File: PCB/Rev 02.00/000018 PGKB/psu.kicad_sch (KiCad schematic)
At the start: 12 parts, among them U6 MCP1825T-3302E/DC, U7 CAT811TTBI-GT3

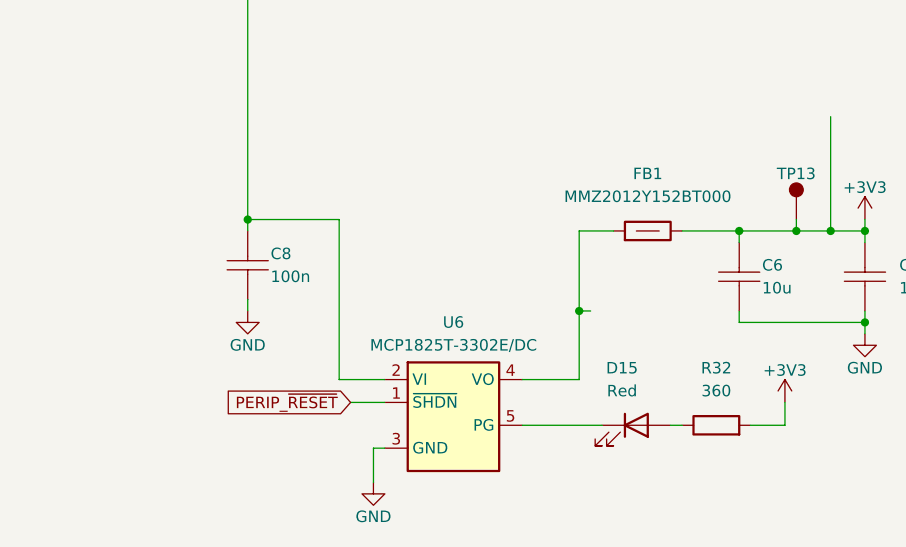
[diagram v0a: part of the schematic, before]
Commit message: Leiskaa
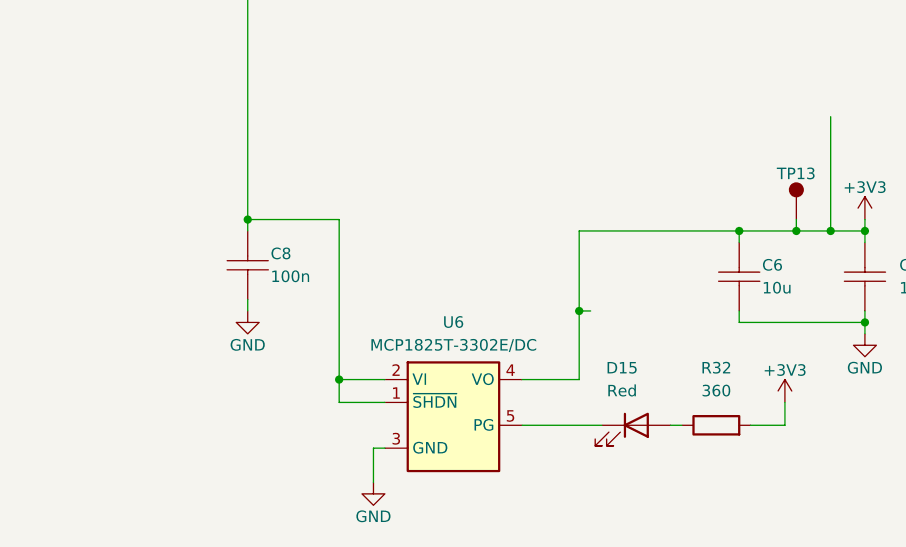
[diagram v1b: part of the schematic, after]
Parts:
- removed FB1: Ferrite_500mA_TDK_MMZ2012Y152BT000, KD_Inductor:INDC2016X100N, symbol KD_Inductor:Ferrite_500mA_TDK_MMZ2012Y152BT000
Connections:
- net +3V3: now also U6.4 (VO)
- net PERIP_~{RESET}: no longer U6.1 (~{SHDN})
- net PWR_IN: now also U6.1 (~{SHDN})
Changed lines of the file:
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@@
   (junction (at 214.63 111.76) (diameter 0) (color 0 0 0 0)
   )
+  (junction (at 81.28 128.27) (diameter 0) (color 0 0 0 0)
+  )
   (junction (at 180.34 111.76) (diameter 0) (color 0 0 0 0)
   )
@@
     (stroke (width 0) (type default))
   )
+  (wire (pts (xy 81.28 130.81) (xy 81.28 128.27))
+    (stroke (width 0) (type default))
+  )
   (wire (pts (xy 81.28 128.27) (xy 86.36 128.27))
     (stroke (width 0) (type default))
@@
     (stroke (width 0) (type default))
   )
-  (wire (pts (xy 82.55 130.81) (xy 86.36 130.81))
+  (wire (pts (xy 81.28 130.81) (xy 86.36 130.81))
     (stroke (width 0) (type default))
   )
@@
     (stroke (width 0) (type default))
   )
-  (wire (pts (xy 119.38 111.76) (xy 125.73 111.76))
-    (stroke (width 0) (type default))
-  )
   (wire (pts (xy 101.6 133.35) (xy 110.49 133.35))
     (stroke (width 0) (type default))
@@
     (stroke (width 0) (type default))
   )
-  (wire (pts (xy 107.95 111.76) (xy 111.76 111.76))
+  (wire (pts (xy 107.95 111.76) (xy 125.73 111.76))
     (stroke (width 0) (type default))
   )
@@
   (wire (pts (xy 139.7 113.03) (xy 139.7 111.76))
     (stroke (width 0) (type default))
-  )
-  (global_label "PERIP_~{RESET}" (shape input) (at 82.55 130.81 180) (fields_autoplaced)
-    (effects (font (size 1.27 1.27)) (justify right))
-    (property "Intersheetrefs" "${INTERSHEET_REFS}" (at 67.1932 130.81 0)
-      (effects (font (size 1.27 1.27)) (justify right) hide)
-    )
   )
   (global_label "PERIP_~{RESET}" (shape output) (at 226.06 111.76 0) (fields_autoplaced)
@@
         )
       )
-    )
-  )
-  (symbol (lib_id "KD_Inductor:Ferrite_500mA_TDK_MMZ2012Y152BT000") (at 115.57 111.76 90) (unit 1)
-    (in_bom yes) (on_board yes) (dnp no) (fields_autoplaced)
-    (property "Reference" "FB1" (at 115.57 105.41 90)
-      (effects (font (size 1.27 1.27)))
-    )
-    (property "Value" "Ferrite_500mA_TDK_MMZ2012Y152BT000" (at 78.74 124.46 0)
-      (effects (font (size 1.27 1.27)) (justify left) hide)
-    )
-    (property "Footprint" "KD_Inductor:INDC2016X100N" (at 96.52 124.46 0)
-      (effects (font (size 1.27 1.27)) (justify left) hide)
-    )
-    (property "Datasheet" "https://product.tdk.com/en/system/files?file=dam/doc/product/emc/emc/beads/catalog/beads_commercial_signal_mmz2012_en.pdf" (at 99.06 124.46 0)
-      (effects (font (size 1.27 1.27)) (justify left) hide)
-    )
-    (property "Code" "MMZ2012Y152BT000" (at 115.57 107.95 90)
-      (effects (font (size 1.27 1.27)))
-    )
-    (property "Manufacturer" "Abracon LLC" (at 81.28 124.46 0)
-      (effects (font (size 1.27 1.27)) (justify left) hide)
-    )
-    (property "MFG_PartNo" "MMZ2012Y152BT000" (at 83.82 124.46 0)
-      (effects (font (size 1.27 1.27)) (justify left) hide)
-    )
-    (property "Supplier" "Digi-Key" (at 86.36 124.46 0)
-      (effects (font (size 1.27 1.27)) (justify left) hide)
-    )
-    (property "Supplier_PartNo" "445-MMZ2012Y152BT000CT-ND" (at 88.9 124.46 0)
-      (effects (font (size 1.27 1.27)) (justify left) hide)
-    )
-    (property "DNP" "F" (at 91.44 124.46 0)
-      (effects (font (size 1.27 1.27)) (justify left) hide)
-    )
-    (property "Price" "0.10" (at 93.98 124.46 0)
-      (effects (font (size 1.27 1.27)) (justify left) hide)
-    )
-    (pin "1")
-    (pin "2")
-    (instances
-      (project "000052 RCCON"
-        (path "/c58960d9-4cac-4036-ad2e-1aef26946dae/eac09b2d-e140-4cbb-8fdb-4c6e8da2411c"
-          (reference "FB1") (unit 1)
-        )
-      )
-      (project "000018 PGKB"
-        (path "/e63e39d7-6ac0-4ffd-8aa3-1841a4541b55/2eb44e1a-4042-4ea6-aca2-4836a6ec84e9/91422aee-53cf-4c28-8efa-7ede5a87a80b"
-          (reference "FB3") (unit 1)
-        )
-      )

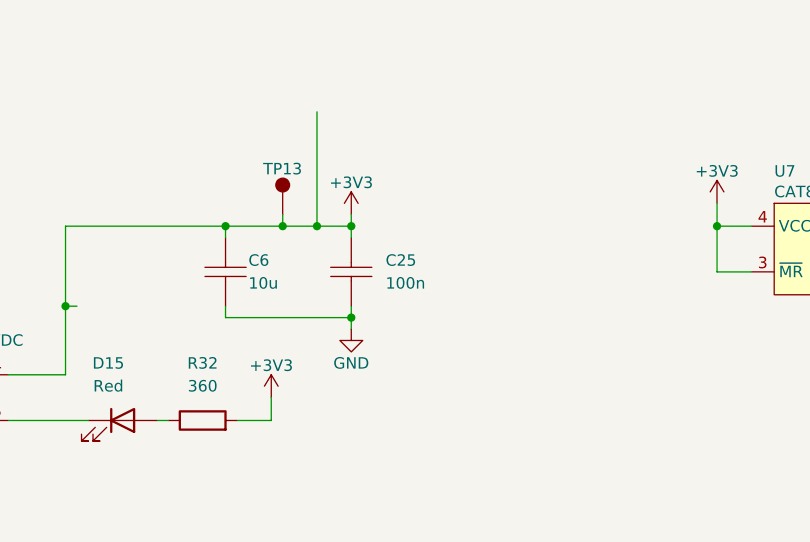
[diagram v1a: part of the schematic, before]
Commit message: error fixing
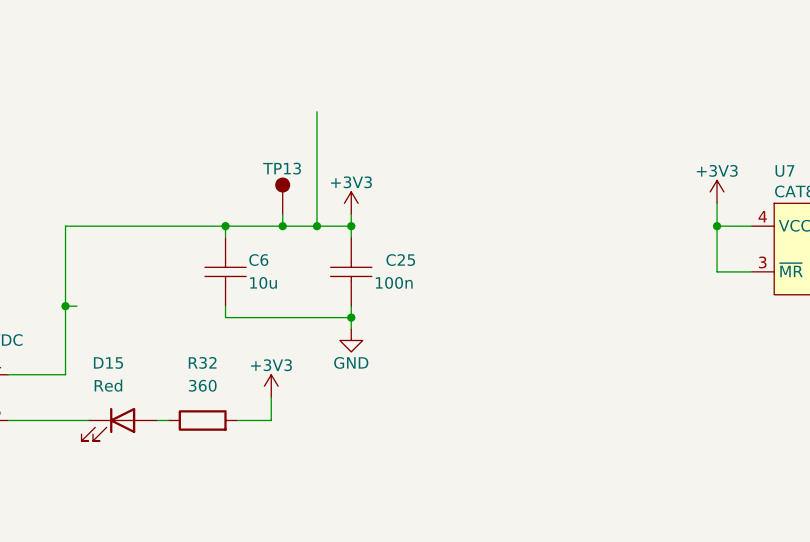
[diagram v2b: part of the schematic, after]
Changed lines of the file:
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@@
   (title_block
     (title "Programmable Keyboard")
-    (date "2023-10-14")
+    (date "2023-10-19")
     (rev "1.0")
     (company "Kallio Designs Oy")
@@
       (effects (font (size 1.27 1.27)) (justify left))
     )
-    (property "Value" "100n" (at 143.51 118.11 0)
+    (property "Value" "100n" (at 142.24 118.11 0)
       (effects (font (size 1.27 1.27)) (justify left))
     )
